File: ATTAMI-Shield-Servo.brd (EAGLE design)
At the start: 22.8 x 22.9 mm, 14 parts

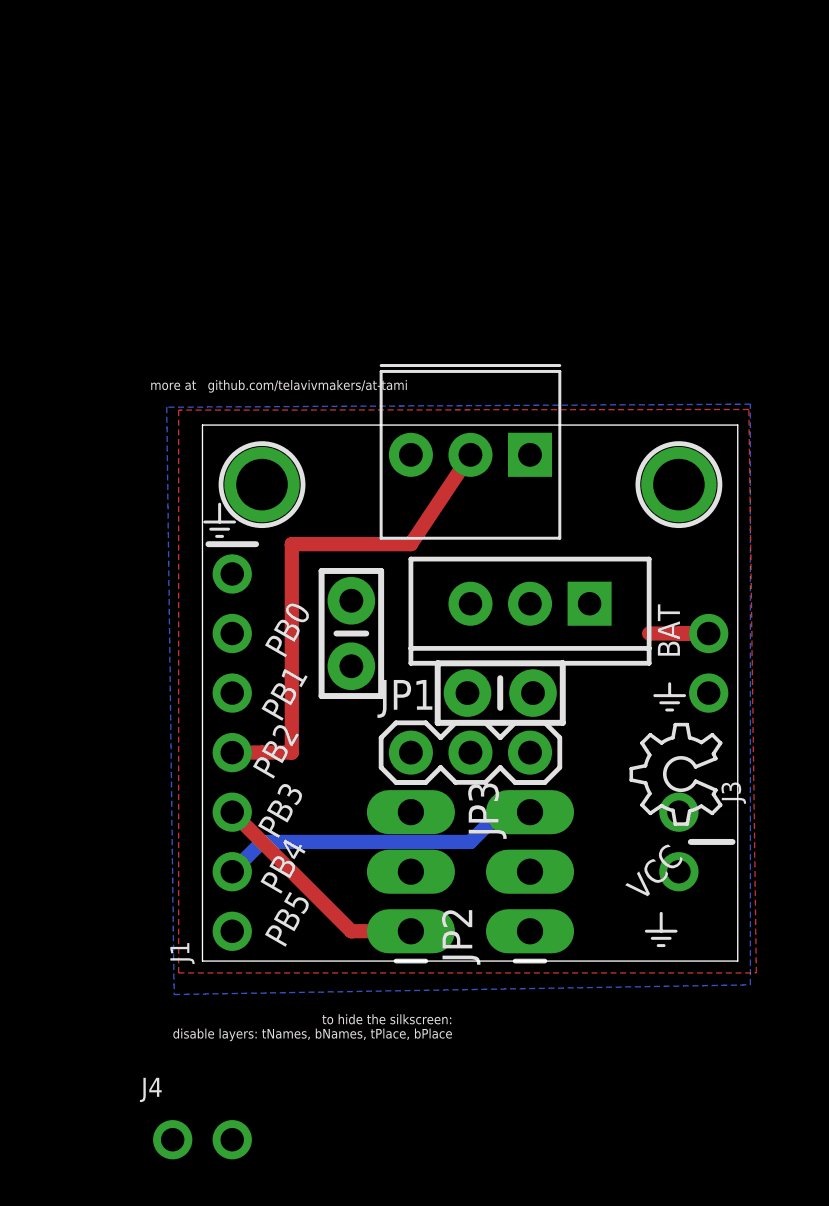
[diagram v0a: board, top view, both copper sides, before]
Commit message: servi inverter
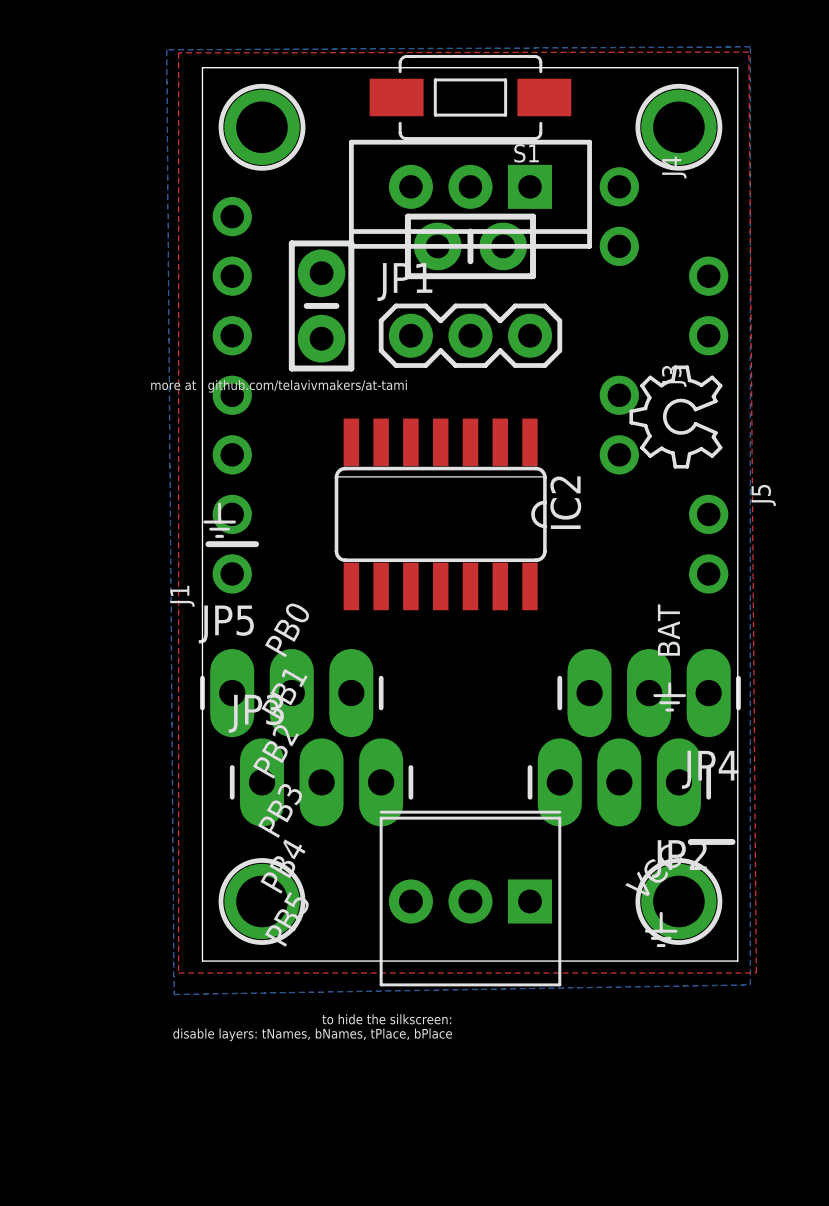
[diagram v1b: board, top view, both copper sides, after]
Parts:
- added IC2: 7404D, 74xx-us:SO14
- added J5: (no value), microbuilder:1X02_ROUND
- added JP4: servo1_mirror, SparkFun-Connectors:1X03_LONGPADS
- added JP5: servo2_mirror, SparkFun-Connectors:1X03_LONGPADS
- added S1: SWITCH-MOMENTARY-2-SMD-1101NE, SparkFun-Electromechanical:TACTILE-SWITCH-1101NE
- added U$4, U$5: MOUNTINGHOLE2.0, microbuilder:MOUNTINGHOLE_2.0_PLATED
- moved J4 43.2 mm to (17.8, 31.8), turned to 270 degrees
- moved C1 19.1 mm to (11.4, 30.5)
- moved POT 19.0 mm to (14.0, 5.08)
- moved IC1 18.0 mm to (11.4, 33.0)
- moved J3 18.0 mm to (17.8, 22.9)
- moved JP1 17.8 mm to (8.89, 26.7)
- moved J2 15.2 mm to (21.6, 27.9)
- moved U$1 15.2 mm to (2.54, 35.6)
- moved U$2 15.2 mm to (20.3, 35.6)
- moved U$3 15.2 mm to (22.1, 21.1)
- moved J1 15.2 mm to (1.27, 24.1)
- moved C2 14.0 mm to (5.08, 27.9)
- moved JP2 8.98 mm to (20.3, 7.62), turned to 180 degrees
- moved JP3 6.48 mm to (2.54, 7.62), turned to 0 degrees
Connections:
- new net N$1: IC2.2, JP4.3
- new net N$5: IC2.4, JP5.3
- net GND: now also IC2.11, IC2.13, IC2.5, IC2.7, IC2.9, J5.2, JP4.1, JP5.1, S1.P$1
- net PB0(MOSI,PWM): now also IC2.1
- net PB1(MISO,PWM): now also IC2.3
- net PB5(RESET): now also S1.P$2
- net VCC: now also IC2.14, J5.1
- net V_BAT: now also JP4.2, JP5.2
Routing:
- net PB2(ADC1\SCK): track 21.1 -> 0.00 mm
- net PB0(MOSI,PWM): track 13.8 -> 0.00 mm
- net PB1(MISO,PWM): track 9.72 -> 0.00 mm
- net V_BAT: track 3.81 -> 0.00 mm
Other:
- board size 22.8 x 22.9 mm -> 22.8 x 38.1 mm

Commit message: servo shield-no invert :(
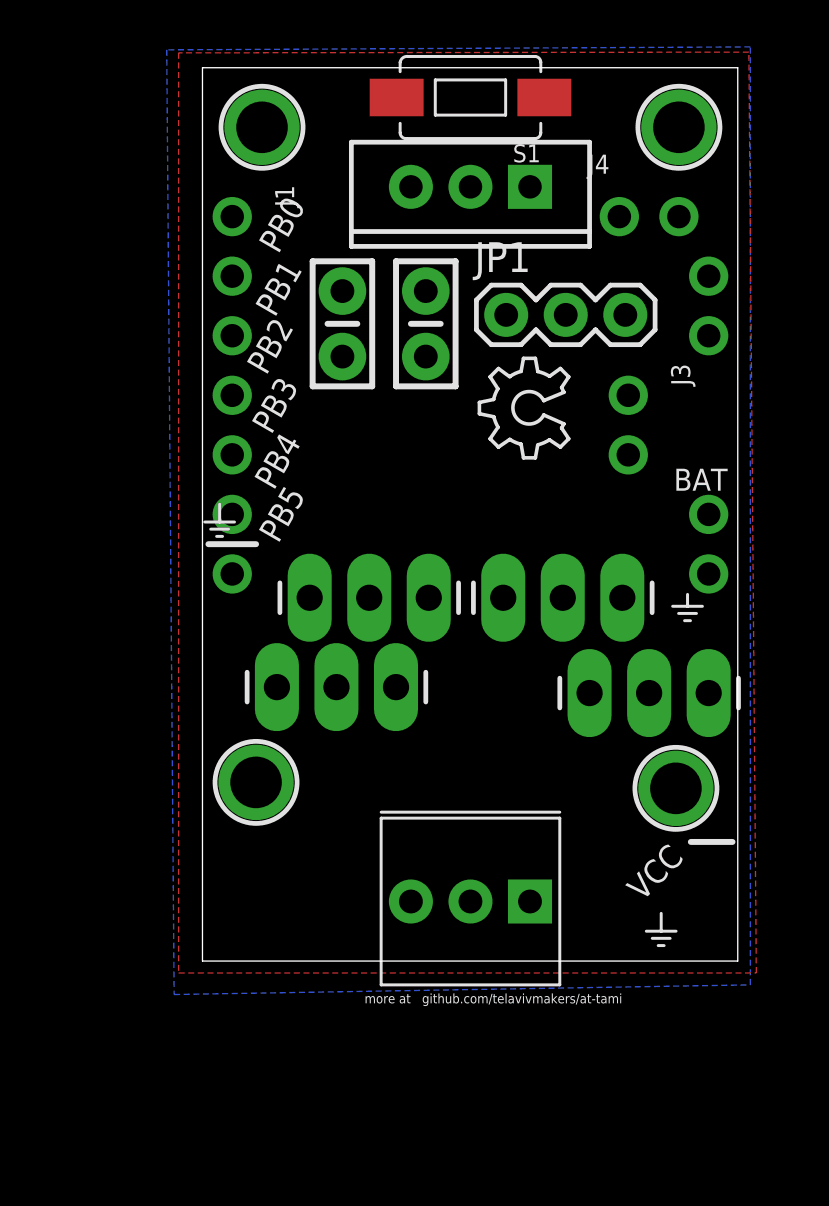
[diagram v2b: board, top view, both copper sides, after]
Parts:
- removed IC2: 7404D, 74xx-us:SO14
- moved JP2 8.24 mm to (17.9, 15.5)
- moved U$3 6.49 mm to (15.6, 21.5)
- moved JP5 5.24 mm to (4.57, 15.5)
- moved U$4 5.09 mm to (2.29, 7.62)
- moved U$5 4.83 mm to (20.2, 7.37)
- moved JP1 4.16 mm to (13.0, 27.6)
- moved JP3 4.11 mm to (3.17, 11.7)
- moved C1 3.81 mm to (9.53, 27.2), turned to 90 degrees
- moved J4 1.27 mm to (19.1, 31.8), turned to 0 degrees
- moved C2 1.17 mm to (5.97, 27.2), turned to 90 degrees
- moved J3 0.38 mm to (18.2, 22.9)
- turned J1 to 270 degrees
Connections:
- removed net N$1: IC2.2, JP4.3
- removed net N$5: IC2.4, JP5.3
- net GND: no longer IC2.11, IC2.13, IC2.5, IC2.7, IC2.9
- net PB0(MOSI,PWM): now also JP4.3; no longer IC2.1
- net PB1(MISO,PWM): now also JP5.3; no longer IC2.3
- net VCC: no longer IC2.14
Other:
- board text removed: "to hide the silkscreen: disable layers: tNames, bNames, tPlace, bPlace"
